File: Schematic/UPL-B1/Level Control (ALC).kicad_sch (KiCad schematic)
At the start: 102 parts, among them P53 TestPoint, P54 TestPoint, P55 TestPoint, P56 TestPoint, P57 TestPoint, P58 TestPoint, X50 Conn_01x03_Pin_Bridge, X51 Conn_01x03_Pin_Bridge, X52 Conn_01x03_Pin_Bridge

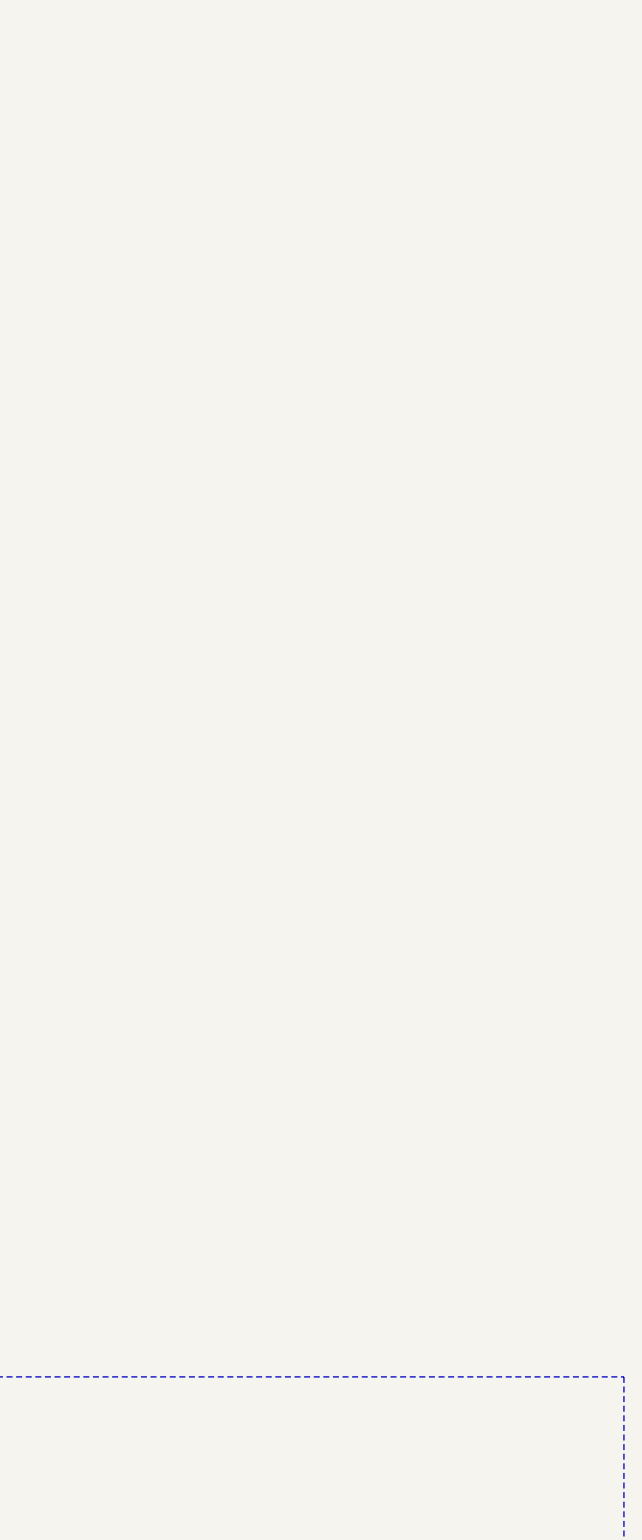
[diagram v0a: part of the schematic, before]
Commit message: Add more expected waveforms
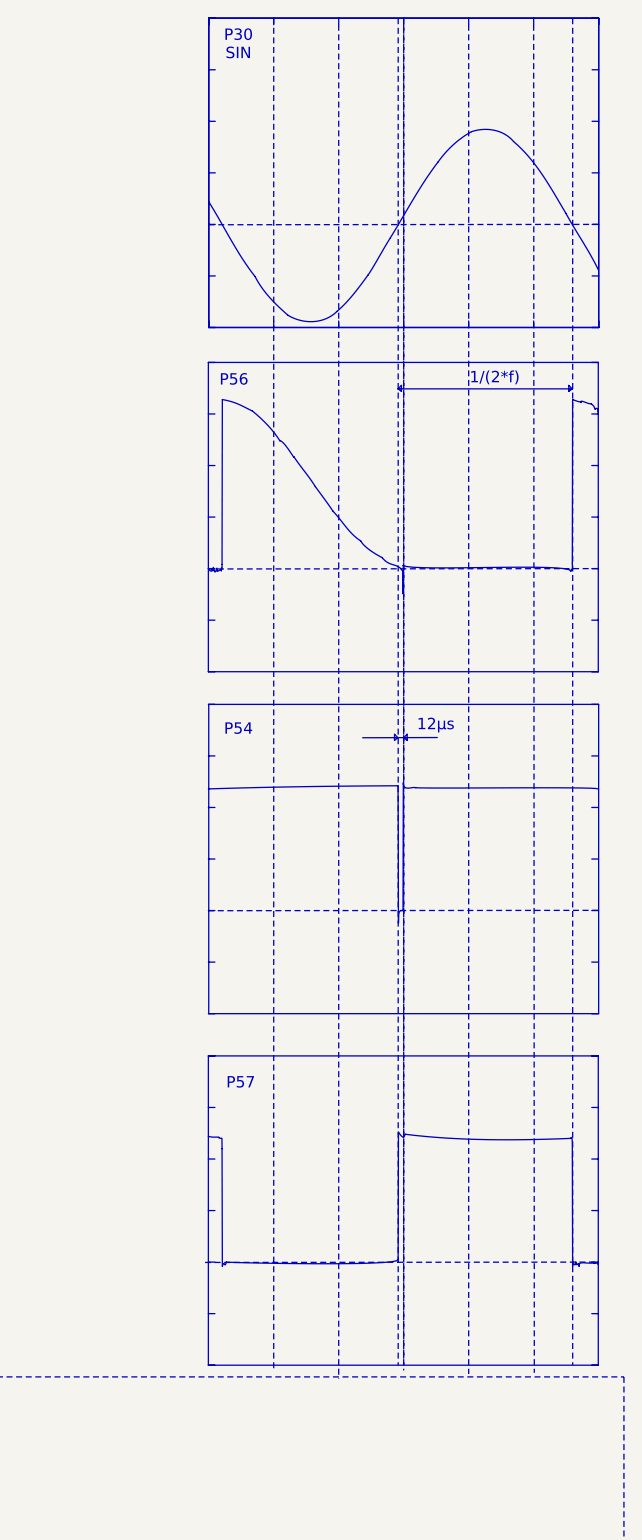
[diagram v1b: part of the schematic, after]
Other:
- note added: "1/(2*f)"
- note added: "12µs"
- note added: "P30 SIN"
- note added: "P54"
- note added: "P56"
- note added: "P57"
